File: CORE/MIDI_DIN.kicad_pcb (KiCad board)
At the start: 2 copper layers, 29.5 x 99.8 mm, 62 parts, among them J1 Conn_02x08_Odd_Even, J2 USB_C_Receptacle_USB2.0, J3 Conn_01x04, J5 MAB5100S, J6 MAB5100S, J7 Conn_01x06, Q1 BSS84, Q2 2N7002, Q5 2N7002, SW1 SW_Slide_SPDT, SW2 SW_Slide_DPDT, SW3 PROG, SW4 SW_DIP_x04, SW5 RST, U1 ATSAMD21G15B-A, U2 H11L1, U3 MIC5504-3.3YM5, U4 MCP2517FD-xSL, U5 MCP2562FD-ESN, Y1 20MHz

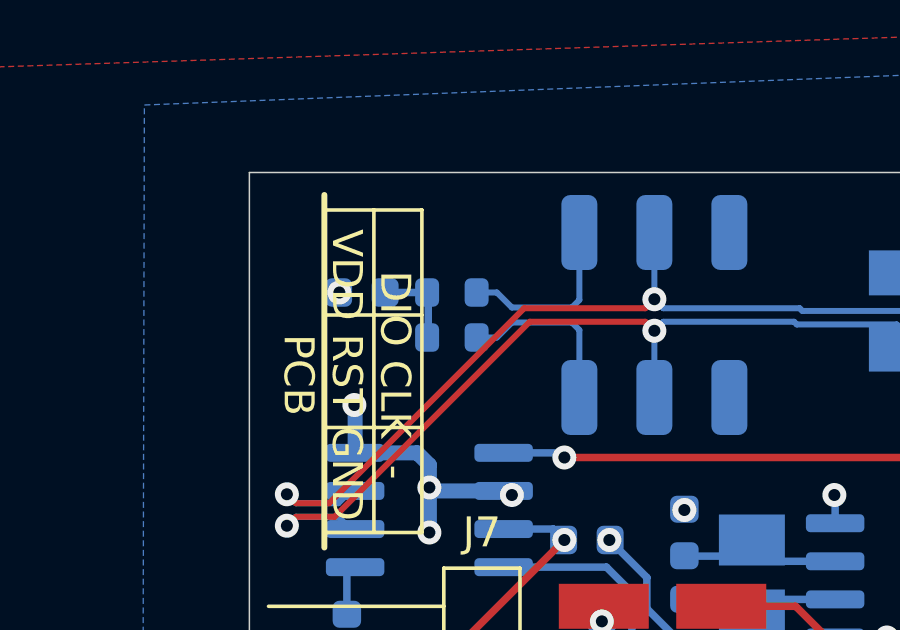
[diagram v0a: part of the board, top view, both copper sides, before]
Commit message: Finalize module
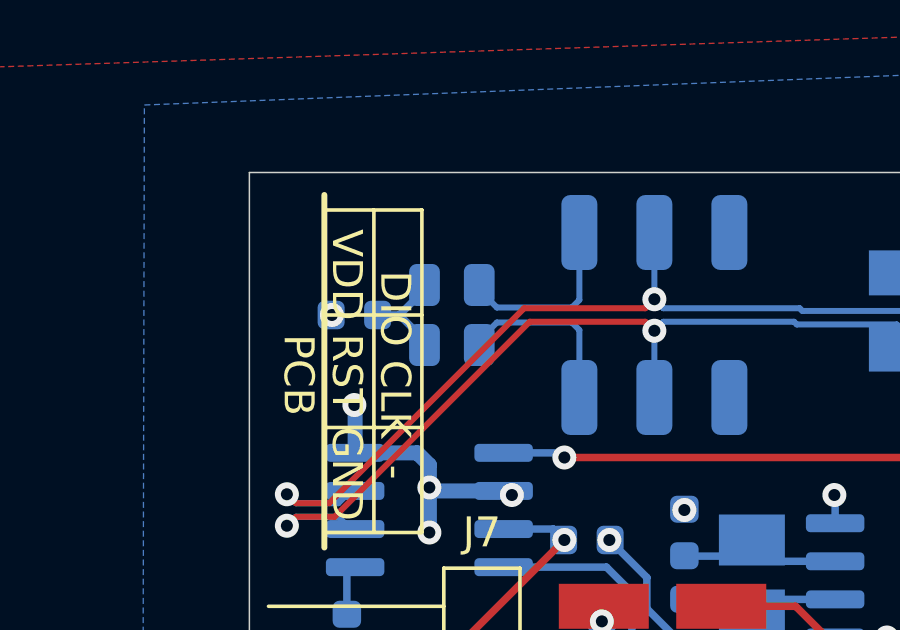
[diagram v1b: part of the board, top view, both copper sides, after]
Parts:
- C13, C14: value 15pF -> 12pF
- R18, R19: footprint Resistor_SMD:R_0603_1608Metric -> Resistor_SMD:R_0805_2012Metric
- moved C16 0.79 mm to (78.8, 50.5)
- moved R18 0.25 mm to (82.0, 49.5)
- moved R19 0.25 mm to (82.0, 51.5)
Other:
- rule pad_to_mask_clearance: 0.05 -> 0
